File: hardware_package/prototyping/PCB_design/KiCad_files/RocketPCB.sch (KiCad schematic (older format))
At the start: 61 parts

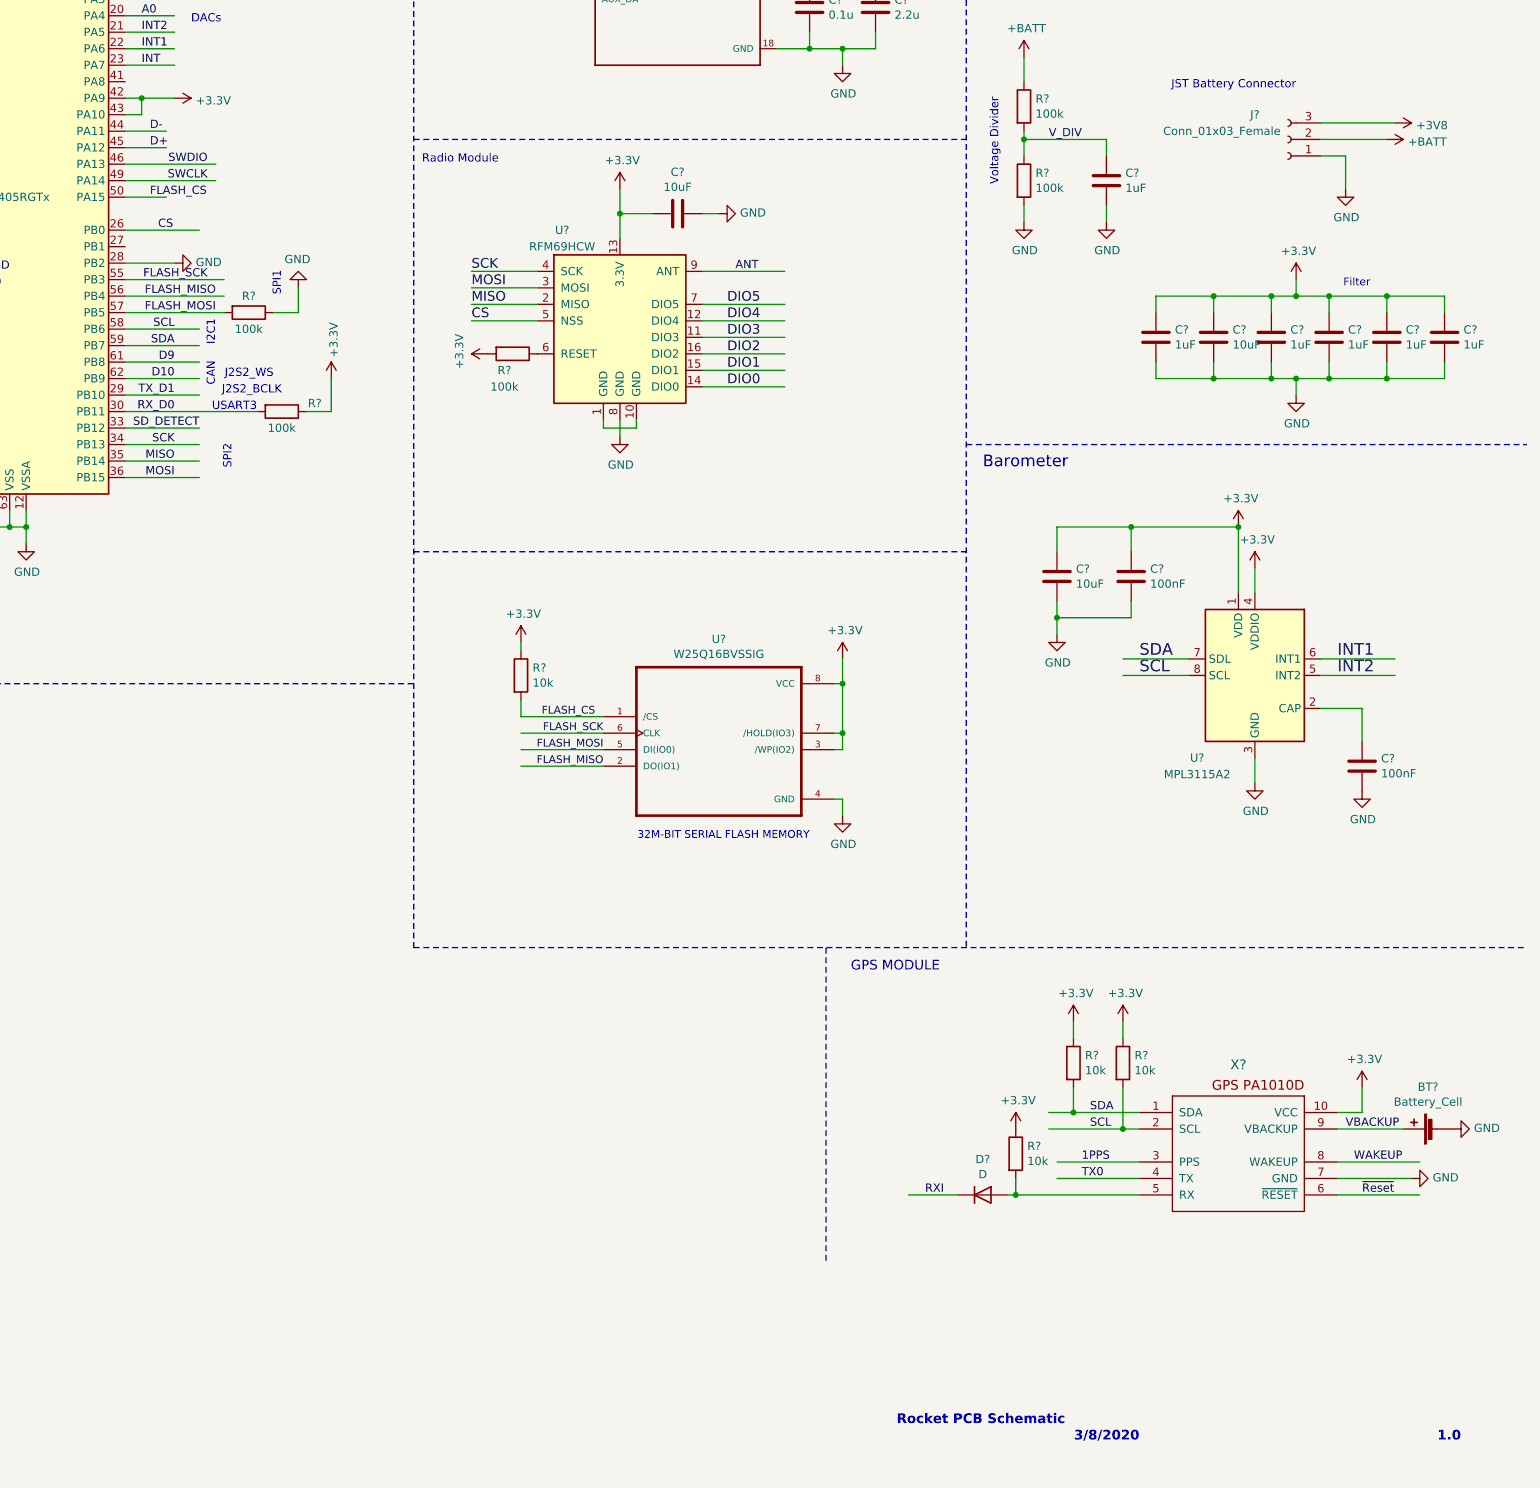
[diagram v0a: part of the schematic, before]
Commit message: Added Battery Regulator
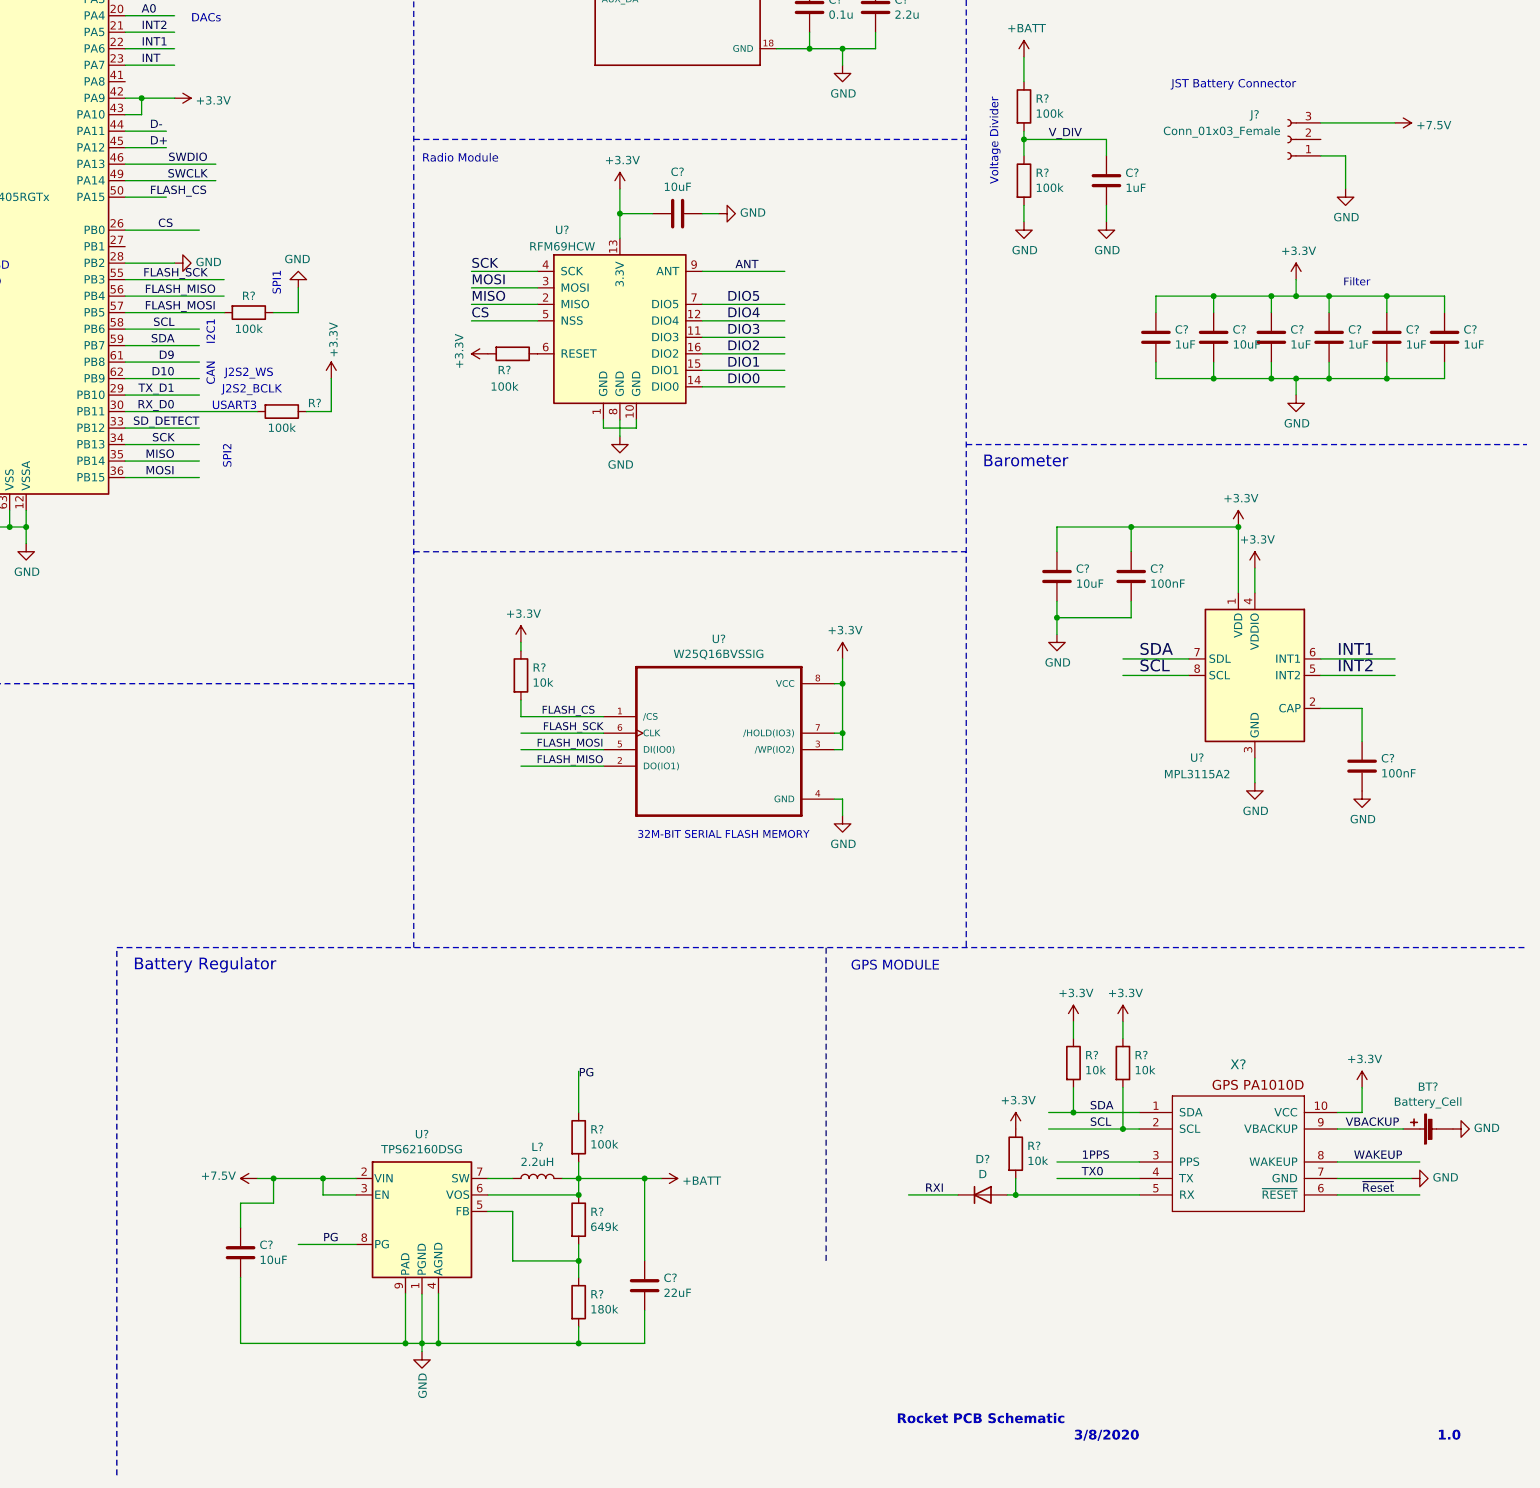
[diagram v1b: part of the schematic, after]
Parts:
- added C?: 22uF, symbol Device:C
- added C?: 10uF, symbol Device:C
- added L?: 2.2uH, symbol Device:L
- added R?: 649k, symbol Device:R
- added R?: 180k, symbol Device:R
- added R?: 100k, symbol Device:R
- added U?: TPS62160DSG, Package_SON:WSON-8-1EP_2x2mm_P0.5mm_EP0.9x1.6mm_ThermalVias, symbol Regulator_Switching:TPS62160DSG
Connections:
- net labels added: +7.5V, PG
- net labels removed: +3V8
- wire segments 290 -> 324
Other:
- note added: "Battery Regulator\n"
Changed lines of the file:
@@
 	-1   0    0    1
 $EndComp
-$Comp
-L power:+BATT #PWR?
-U 1 1 5F51DC94
-P 15200 3150
-F 0 "#PWR?" H 15200 3000 50  0001 C CNN
-F 1 "+BATT" V 15215 3278 50  0000 L CNN
-F 2 "" H 15200 3150 50  0001 C CNN
-F 3 "" H 15200 3150 50  0001 C CNN
-	1    15200 3150
-	0    1    1    0
-$EndComp
-Wire Wire Line
-	14800 3150 15200 3150
 Wire Wire Line
 	14800 3250 14950 3250
@@
 	12650 500  12650 8050
 Wire Notes Line
-	9300 8050 16050 8050
-Wire Notes Line
 	9300 450  9300 8050
 Text Label 13150 3150 0    50   ~ 0
@@
 Wire Wire Line
 	14800 3050 15250 3050
-$Comp
-L power:+3V8 #PWR?
-U 1 1 5F95B0D5
-P 15250 3050
-F 0 "#PWR?" H 15250 2900 50  0001 C CNN
-F 1 "+3V8" V 15265 3178 50  0000 L CNN
-F 2 "" H 15250 3050 50  0001 C CNN
-F 3 "" H 15250 3050 50  0001 C CNN
-	1    15250 3050
-	0    1    1    0
-$EndComp
 Wire Wire Line
 	7550 3700 8000 3700
@@
 Text Notes 2500 3950 0    71   ~ 0
 Reset & Prog Switches\n
+$Comp
+L Regulator_Switching:TPS62160DSG U?
+U 1 1 5F72D5C8
+P 9350 9750
+F 0 "U?" H 9350 10317 50  0000 C CNN
+F 1 "TPS62160DSG" H 9350 10226 50  0000 C CNN
+F 2 "Package_SON:WSON-8-1EP_2x2mm_P0.5mm_EP0.9x1.6mm_ThermalVias" H 9500 9400 50  0001 L CNN
+F 3 "http://www.ti.com/lit/ds/symlink/tps62160.pdf" H 9350 10300 50  0001 C CNN
+	1    9350 9750
+	1    0    0    -1
+$EndComp
+$Comp
+L power:+7.5V #PWR?
+U 1 1 5F74C0CF
+P 15250 3050
+F 0 "#PWR?" H 15250 2900 50  0001 C CNN
+F 1 "+7.5V" V 15265 3178 50  0000 L CNN
+F 2 "" H 15250 3050 50  0001 C CNN
+F 3 "" H 15250 3050 50  0001 C CNN
+	1    15250 3050
+	0    1    1    0
+$EndComp
+$Comp
+L power:+7.5V #PWR?
+U 1 1 5F7502B8
+P 8350 9450
+F 0 "#PWR?" H 8350 9300 50  0001 C CNN
+F 1 "+7.5V" V 8365 9578 50  0000 L CNN
+F 2 "" H 8350 9450 50  0001 C CNN
+F 3 "" H 8350 9450 50  0001 C CNN
+	1    8350 9450
+	0    -1   -1   0
+$EndComp
+Wire Wire Line
+	8350 9450 8450 9450
+Wire Wire Line
+	8950 9550 8750 9550
+Wire Wire Line
+	8750 9550 8750 9450
+Connection ~ 8750 9450
+Wire Wire Line
+	8750 9450 8950 9450
+$Comp
+L Device:L L?
+U 1 1 5F7CC9EF
+P 10050 9450
+F 0 "L?" V 10240 9450 50  0000 C CNN
+F 1 "2.2uH" V 10149 9450 50  0000 C CNN
+F 2 "" H 10050 9450 50  0001 C CNN
+F 3 "~" H 10050 9450 50  0001 C CNN
+	1    10050 9450
+	0    -1   -1   0
+$EndComp
+Wire Wire Line
+	9750 9450 9900 9450
+Wire Wire Line
+	9750 9550 10300 9550
+Wire Wire Line
+	10300 9550 10300 9450
+Wire Wire Line
+	10300 9450 10200 9450
+$Comp
+L Device:R R?
+U 1 1 5F8016AA
+P 10300 9700
+F 0 "R?" H 10370 9746 50  0000 L CNN
+F 1 "649k" H 10370 9655 50  0000 L CNN
+F 2 "" V 10230 9700 50  0001 C CNN
+F 3 "~" H 10300 9700 50  0001 C CNN
+	1    10300 9700
+	1    0    0    -1
+$EndComp
+Connection ~ 10300 9550
+Wire Wire Line
+	10300 9850 10300 9950
+Wire Wire Line
+	10300 9950 9900 9950
+Wire Wire Line
+	9900 9950 9900 9650
+Wire Wire Line
+	9900 9650 9750 9650
+Wire Wire Line
+	10300 9950 10300 10050
+Connection ~ 10300 9950
+$Comp
+L Device:R R?
+U 1 1 5F8384B0
+P 10300 10200
+F 0 "R?" H 10370 10246 50  0000 L CNN
+F 1 "180k" H 10370 10155 50  0000 L CNN
+F 2 "" V 10230 10200 50  0001 C CNN
+F 3 "~" H 10300 10200 50  0001 C CNN
+	1    10300 10200
+	1    0    0    -1
+$EndComp
+Wire Wire Line
+	10300 10350 10300 10450
+Wire Wire Line
+	10300 10450 9450 10450
+Wire Wire Line
+	10300 9450 10700 9450
+Wire Wire Line
+	10700 9450 10700 9950
+Connection ~ 10300 9450
+$Comp
+L Device:C C?
+U 1 1 5F8702D4
+P 10700 10100
+F 0 "C?" H 10815 10146 50  0000 L CNN
+F 1 "22uF" H 10815 10055 50  0000 L CNN
+F 2 "" H 10738 9950 50  0001 C CNN
+F 3 "~" H 10700 10100 50  0001 C CNN
+	1    10700 10100
+	1    0    0    -1
+$EndComp
+Wire Wire Line
+	10700 10250 10700 10450
+Wire Wire Line
+	10700 10450 10300 10450
+Connection ~ 10300 10450
+Wire Wire Line
+	10700 9450 10800 9450
+Connection ~ 10700 9450
+$Comp
+L Device:C C?
+U 1 1 5F8E3FA7
+P 8250 9900
+F 0 "C?" H 8365 9946 50  0000 L CNN
+F 1 "10uF" H 8365 9855 50  0000 L CNN
+F 2 "" H 8288 9750 50  0001 C CNN
+F 3 "~" H 8250 9900 50  0001 C CNN
+	1    8250 9900
+	1    0    0    -1
+$EndComp
+Wire Wire Line
+	8450 9450 8450 9600
+Wire Wire Line
+	8450 9600 8250 9600
+Wire Wire Line
+	8250 9600 8250 9750
+Connection ~ 8450 9450
+Wire Wire Line
+	8450 9450 8750 9450
+Text Label 8750 9850 0    50   ~ 0
+PG
+Wire Wire Line
+	8950 9850 8600 9850
+$Comp
+L Device:R R?
+U 1 1 5F983424
+P 10300 9200
+F 0 "R?" H 10370 9246 50  0000 L CNN
+F 1 "100k" H 10370 9155 50  0000 L CNN
+F 2 "" V 10230 9200 50  0001 C CNN
+F 3 "~" H 10300 9200 50  0001 C CNN
+	1    10300 9200
+	1    0    0    -1
+$EndComp
+Wire Wire Line
+	10300 9450 10300 9350
+Wire Wire Line
+	10300 9050 10300 8800
+Text Label 10300 8850 0    50   ~ 0
+PG
+$Comp
+L power:+BATT #PWR?
+U 1 1 5F9BFCD8
+P 10800 9450
+F 0 "#PWR?" H 10800 9300 50  0001 C CNN
+F 1 "+BATT" V 10815 9578 50  0000 L CNN
+F 2 "" H 10800 9450 50  0001 C CNN
+F 3 "" H 10800 9450 50  0001 C CNN
+	1    10800 9450
+	0    1    1    0
+$EndComp
+Wire Wire Line
+	9450 10150 9450 10450
+Wire Wire Line
+	9350 10150 9350 10450
+Wire Wire Line
+	9350 10450 9450 10450
+Connection ~ 9450 10450
+Wire Wire Line
+	9250 10150 9250 10450
+Wire Wire Line
+	9250 10450 9350 10450
+Connection ~ 9350 10450
+Wire Wire Line
+	8250 10450 9250 10450
+Wire Wire Line
+	8250 10050 8250 10450
+Connection ~ 9250 10450
+Wire Wire Line
+	9350 10450 9350 10500
+$Comp
+L power:GND #PWR?
+U 1 1 5FA693A7
+P 9350 10500
+F 0 "#PWR?" H 9350 10250 50  0001 C CNN
+F 1 "GND" V 9355 10372 50  0000 R CNN
+F 2 "" H 9350 10500 50  0001 C CNN
+F 3 "" H 9350 10500 50  0001 C CNN
+	1    9350 10500
+	1    0    0    -1
+$EndComp
+Wire Notes Line
+	7500 11250 7500 8050
+Wire Notes Line
+	7500 8050 16050 8050
+Text Notes 7600 8200 0    71   ~ 0
+Battery Regulator\n
 $EndSCHEMATC
